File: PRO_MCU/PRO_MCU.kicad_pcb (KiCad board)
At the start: 2 copper layers, 80 x 41 mm, 21 parts, among them Q1 TN0702, Q2 TN0702, U1 Chassis, U2 ItsyBitsy_NRF52840, U3 MPRLS, U4 Buttons_LED, U5 waveshare_15867

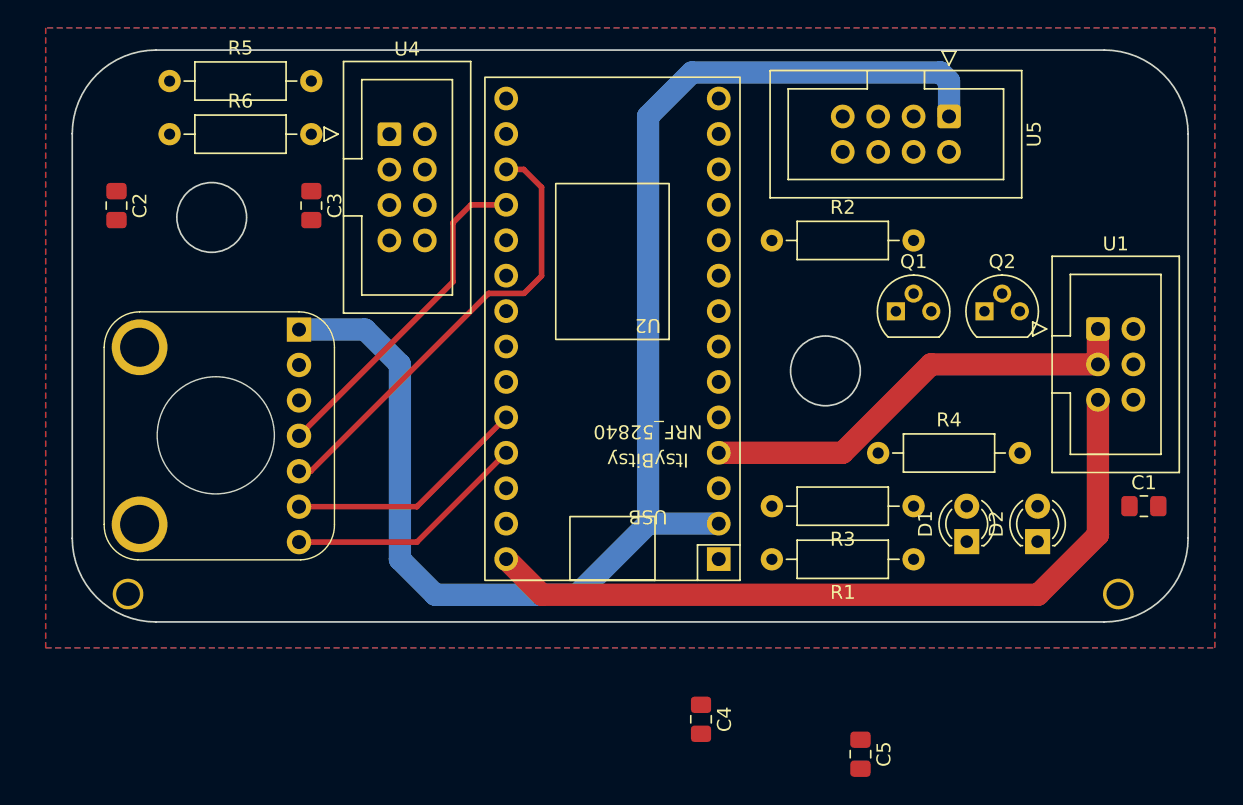
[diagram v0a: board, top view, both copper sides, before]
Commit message: V1.0 Fabrication
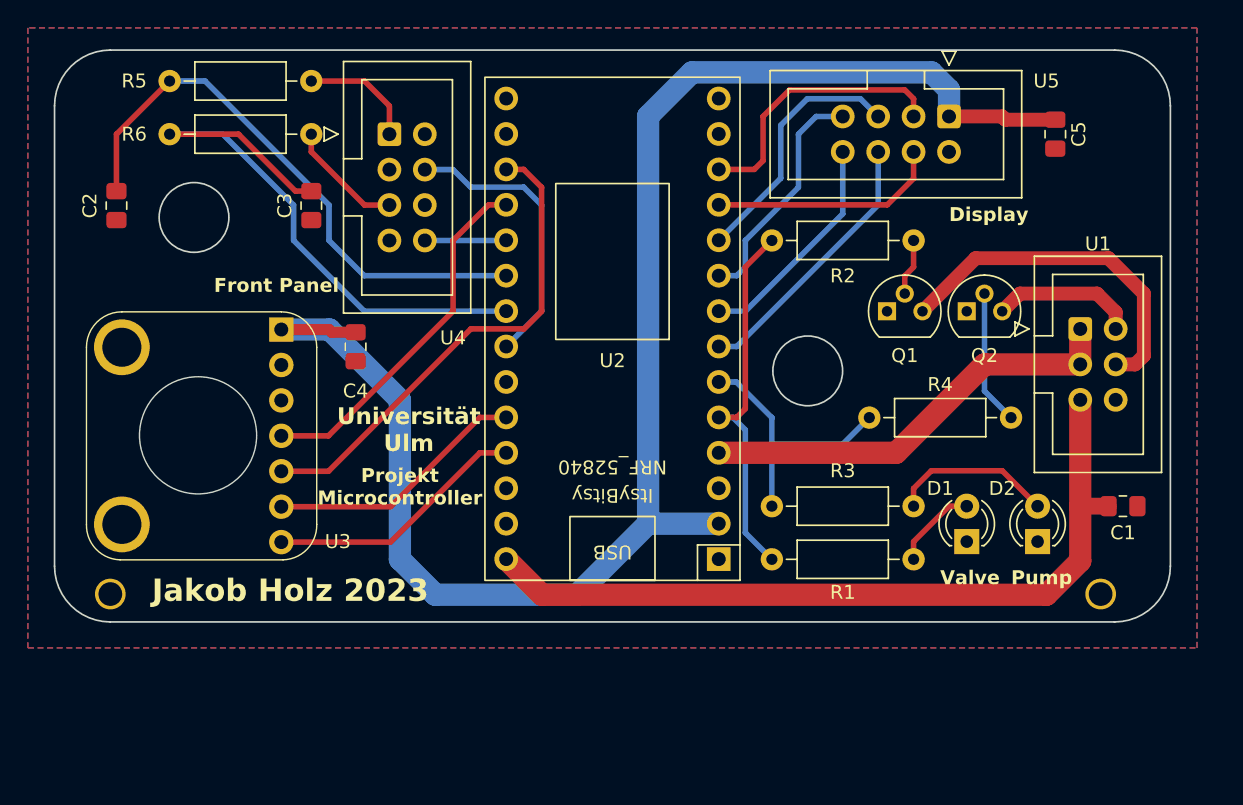
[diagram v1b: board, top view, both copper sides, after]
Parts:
- removed the Logo at (-341.6, 110.5)
- added Logo: BoardGeometry, PRO_MCU:BoardGeometry, F.Cu at (-342.9, 110.5)
- moved C5 46.6 mm to (-311.1, 96.5)
- moved C4 36.4 mm to (-361.3, 111.8)
- moved R4 2.62 mm to (-324.5, 116.8)
- moved C1 1.50 mm to (-306.3, 123.2)
- moved U1 1.27 mm to (-309.4, 110.5)
- moved U3 1.27 mm to (-372.1, 118.1)
- moved Q2 1.27 mm to (-317.5, 109.2)
- moved Q1 0.63 mm to (-323.2, 109.2)
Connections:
- U2 pad 10: /DC -> /CS
- U2 pad 7: /BL -> /DC
- U2 pad 8: /Display_RESET -> /BL
- U2 pad 9: /CS -> /Display_RESET
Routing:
- net /Button_Red: track 0.00 -> 42.7 mm
- net /Button_Green: track 0.00 -> 40.9 mm
- net /Valve_Ctrl: track 0.00 -> 27.4 mm
- net /Valve-: track 0.00 -> 25.2 mm
- net /Led_Green: track 0.00 -> 20.6 mm
- net /MOSI: track 0.00 -> 19.7 mm
- net /DC: track 0.00 -> 19.4 mm
- net /Pump_Ctrl: track 0.00 -> 19.0 mm
- net /CS: track 0.00 -> 18.4 mm
- net /Display_RESET: track 0.00 -> 17.0 mm
- net /SCK: track 0.00 -> 16.7 mm
- net /BL: track 0.00 -> 16.2 mm
- net +3.3V: track 103.1 -> 115.7 mm
- net Net-(D2-A): track 0.00 -> 11.7 mm
- net /Pump-: track 0.00 -> 10.4 mm
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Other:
- outline, holes or cut-outs redrawn
- board text added: "Display"
- board text added: "Front Panel"
- board text added: "Jakob Holz 2023"
- board text added: "Projekt Microcontroller"
- board text added: "Pump"
- board text added: "Universität Ulm"
- board text added: "Valve"
